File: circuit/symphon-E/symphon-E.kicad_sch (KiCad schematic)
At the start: 1 part

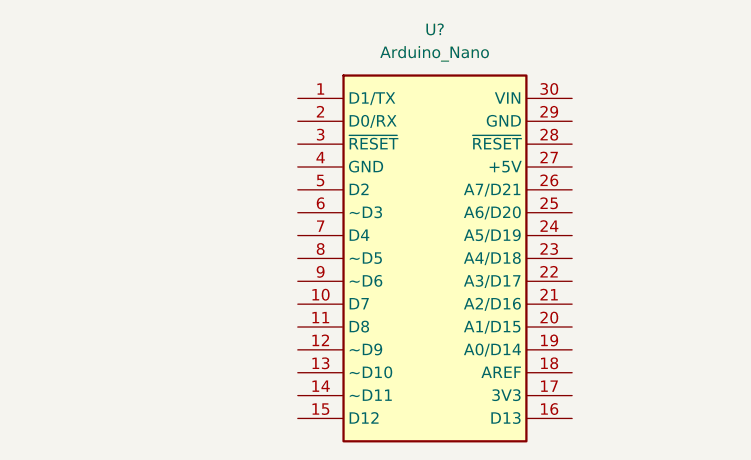
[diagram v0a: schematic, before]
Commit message: add pinout
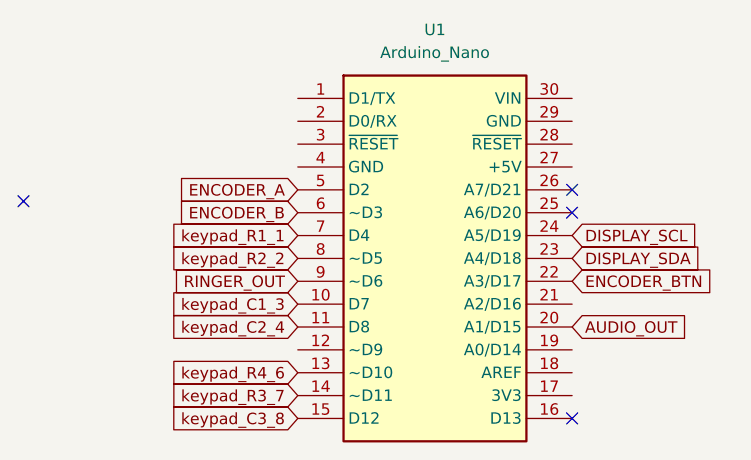
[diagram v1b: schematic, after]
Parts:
- gave numbers to parts that had none: 1
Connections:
- net keypad_C1_3: now reaches U1.10 (D7)
- net keypad_C2_4: now reaches U1.11 (D8)
- net keypad_R4_6: now reaches U1.13 (~D10)
- net keypad_R3_7: now reaches U1.14 (~D11)
- net keypad_C3_8: now reaches U1.15 (D12)
- net AUDIO_OUT: now reaches U1.20 (A1/D15)
- net ENCODER_BTN: now reaches U1.22 (A3/D17)
- net DISPLAY_SDA: now reaches U1.23 (A4/D18)
- net DISPLAY_SCL: now reaches U1.24 (A5/D19)
- net ENCODER_A: now reaches U1.5 (D2)
- net ENCODER_B: now reaches U1.6 (~D3)
- net keypad_R1_1: now reaches U1.7 (D4)
- net keypad_R2_2: now reaches U1.8 (~D5)
- net RINGER_OUT: now reaches U1.9 (~D6)
- no-connect marks 0 -> 4
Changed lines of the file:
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@@
 (kicad_sch (version 20211123) (generator eeschema)
   (paper "A4")
+  (no_connect (at 69.85 44.45))
+  (no_connect (at 8.89 43.18))
+  (no_connect (at 69.85 67.31))
+  (no_connect (at 69.85 41.91))
+  (global_label "ENCODER_A" (shape input) (at 39.37 41.91 180) (fields_autoplaced)
+    (effects (font (size 1.27 1.27)) (justify right))
+    (property "Intersheet References" "${INTERSHEET_REFS}" (id 0) (at 26.1317 41.8306 0)
+      (effects (font (size 1.27 1.27)) (justify right) hide)
+    )
+  )
+  (global_label "keypad_R2_2" (shape input) (at 39.37 49.53 180) (fields_autoplaced)
+    (effects (font (size 1.27 1.27)) (justify right))
+    (property "Intersheet References" "${INTERSHEET_REFS}" (id 0) (at 24.8012 49.4506 0)
+      (effects (font (size 1.27 1.27)) (justify right) hide)
+    )
+  )
+  (global_label "keypad_R4_6" (shape input) (at 39.37 62.23 180) (fields_autoplaced)
+    (effects (font (size 1.27 1.27)) (justify right))
+    (property "Intersheet References" "${INTERSHEET_REFS}" (id 0) (at 24.8012 62.1506 0)
+      (effects (font (size 1.27 1.27)) (justify right) hide)
+    )
+  )
+  (global_label "keypad_C2_4" (shape input) (at 39.37 57.15 180) (fields_autoplaced)
+    (effects (font (size 1.27 1.27)) (justify right))
+    (property "Intersheet References" "${INTERSHEET_REFS}" (id 0) (at 24.8012 57.0706 0)
+      (effects (font (size 1.27 1.27)) (justify right) hide)
+    )
+  )
+  (global_label "DISPLAY_SCL" (shape input) (at 69.85 46.99 0) (fields_autoplaced)
+    (effects (font (size 1.27 1.27)) (justify left))
+    (property "Intersheet References" "${INTERSHEET_REFS}" (id 0) (at 84.2979 46.9106 0)
+      (effects (font (size 1.27 1.27)) (justify left) hide)
+    )
+  )
+  (global_label "DISPLAY_SDA" (shape input) (at 69.85 49.53 0) (fields_autoplaced)
+    (effects (font (size 1.27 1.27)) (justify left))
+    (property "Intersheet References" "${INTERSHEET_REFS}" (id 0) (at 84.3583 49.4506 0)
+      (effects (font (size 1.27 1.27)) (justify left) hide)
+    )
+  )
+  (global_label "keypad_R1_1" (shape input) (at 39.37 46.99 180) (fields_autoplaced)
+    (effects (font (size 1.27 1.27)) (justify right))
+    (property "Intersheet References" "${INTERSHEET_REFS}" (id 0) (at 24.8012 46.9106 0)
+      (effects (font (size 1.27 1.27)) (justify right) hide)
+    )
+  )
+  (global_label "RINGER_OUT" (shape input) (at 39.37 52.07 180) (fields_autoplaced)
+    (effects (font (size 1.27 1.27)) (justify right))
+    (property "Intersheet References" "${INTERSHEET_REFS}" (id 0) (at 25.4664 51.9906 0)
+      (effects (font (size 1.27 1.27)) (justify right) hide)
+    )
+  )
+  (global_label "keypad_C1_3" (shape input) (at 39.37 54.61 180) (fields_autoplaced)
+    (effects (font (size 1.27 1.27)) (justify right))
+    (property "Intersheet References" "${INTERSHEET_REFS}" (id 0) (at 24.8012 54.5306 0)
+      (effects (font (size 1.27 1.27)) (justify right) hide)
+    )
+  )
+  (global_label "AUDIO_OUT" (shape input) (at 69.85 57.15 0) (fields_autoplaced)
+    (effects (font (size 1.27 1.27)) (justify left))
+    (property "Intersheet References" "${INTERSHEET_REFS}" (id 0) (at 82.4836 57.0706 0)
+      (effects (font (size 1.27 1.27)) (justify left) hide)
+    )
+  )
+  (global_label "ENCODER_B" (shape input) (at 39.37 44.45 180) (fields_autoplaced)
+    (effects (font (size 1.27 1.27)) (justify right))
+    (property "Intersheet References" "${INTERSHEET_REFS}" (id 0) (at 25.9502 44.3706 0)
+      (effects (font (size 1.27 1.27)) (justify right) hide)
+    )
+  )
+  (global_label "ENCODER_BTN" (shape input) (at 69.85 52.07 0) (fields_autoplaced)
+    (effects (font (size 1.27 1.27)) (justify left))
+    (property "Intersheet References" "${INTERSHEET_REFS}" (id 0) (at 85.5679 51.9906 0)
+      (effects (font (size 1.27 1.27)) (justify left) hide)
+    )
+  )
+  (global_label "keypad_R3_7" (shape input) (at 39.37 64.77 180) (fields_autoplaced)
+    (effects (font (size 1.27 1.27)) (justify right))
+    (property "Intersheet References" "${INTERSHEET_REFS}" (id 0) (at 24.8012 64.6906 0)
+      (effects (font (size 1.27 1.27)) (justify right) hide)
+    )
+  )
+  (global_label "keypad_C3_8" (shape input) (at 39.37 67.31 180) (fields_autoplaced)
+    (effects (font (size 1.27 1.27)) (justify right))
+    (property "Intersheet References" "${INTERSHEET_REFS}" (id 0) (at 24.8012 67.2306 0)
+      (effects (font (size 1.27 1.27)) (justify right) hide)
+    )
+  )
   (symbol (lib_id "Arduino:Arduino_Nano") (at 54.61 49.53 0) (unit 1)
     (in_bom yes) (on_board yes) (fields_autoplaced)
-    (property "Reference" "U?" (id 0) (at 54.61 24.13 0))
+    (property "Reference" "U1" (id 0) (at 54.61 24.13 0))
     (property "Value" "Arduino_Nano" (id 1) (at 54.61 26.67 0))
     (property "Footprint" "Arduino:Arduino_Nano" (id 2) (at 54.61 71.12 0)
@@
   (symbol_instances
     (path "/05df8035-1ae4-4fd6-8683-6c4f92e2cd4b"
-      (reference "U?") (unit 1) (value "Arduino_Nano") (footprint "Arduino:Arduino_Nano")
+      (reference "U1") (unit 1) (value "Arduino_Nano") (footprint "Arduino:Arduino_Nano")
     )
   )

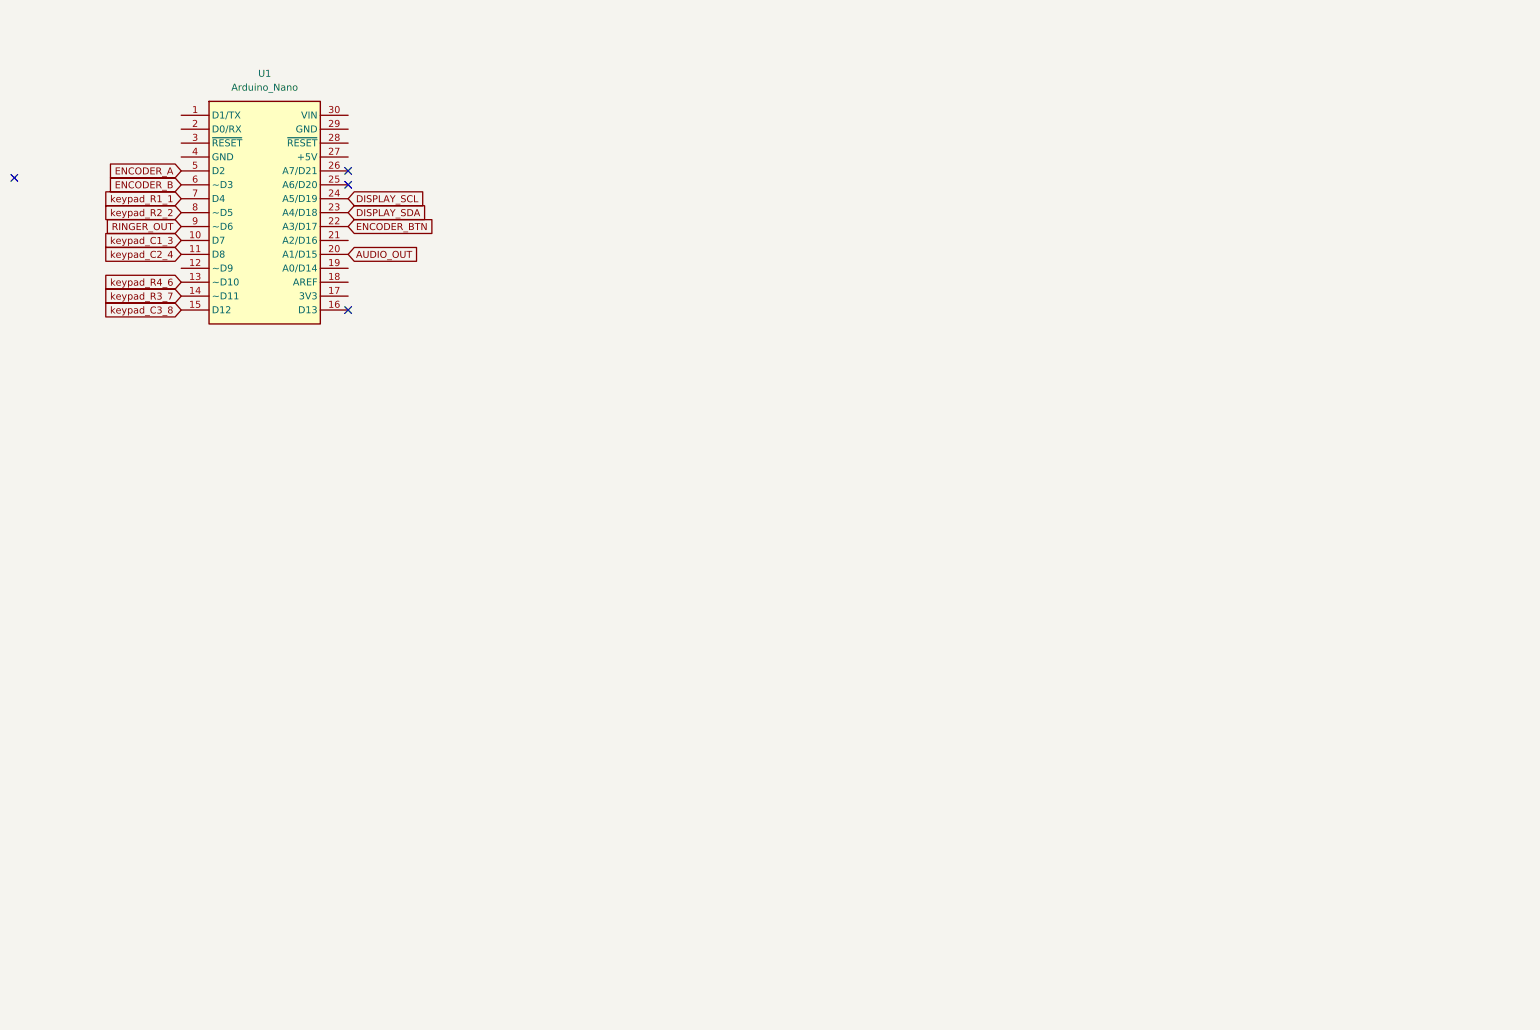
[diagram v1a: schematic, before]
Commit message: add pcb
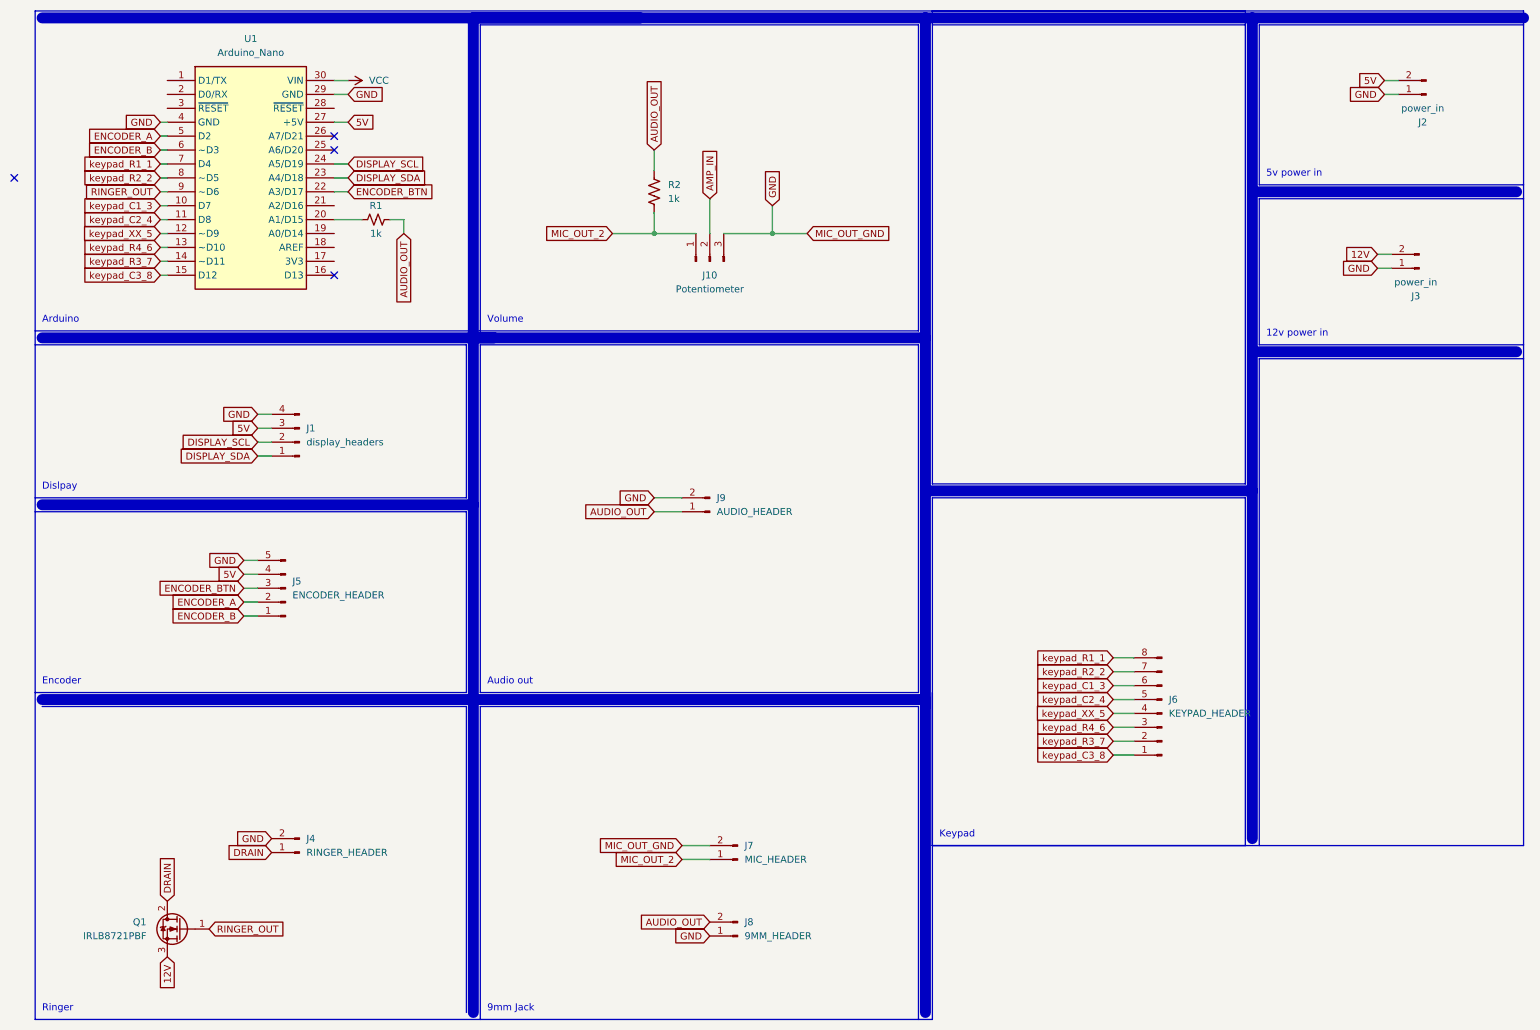
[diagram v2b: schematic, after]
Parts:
- added J1: display_headers, Connector_JST:JST_EH_B4B-EH-A_1x04_P2.50mm_Vertical, symbol Connector:Conn_01x04_Male
- added J10: Potentiometer, Connector_JST:JST_EH_B3B-EH-A_1x03_P2.50mm_Vertical, symbol Connector:Conn_01x03_Male
- added J2, J3: power_in, Connector_JST:JST_EH_B2B-EH-A_1x02_P2.50mm_Vertical, symbol Connector:Conn_01x02_Male
- added J4: RINGER_HEADER, Connector_JST:JST_EH_B2B-EH-A_1x02_P2.50mm_Vertical, symbol Connector:Conn_01x02_Male
- added J5: ENCODER_HEADER, Connector_JST:JST_EH_B5B-EH-A_1x05_P2.50mm_Vertical, symbol Connector:Conn_01x05_Male
- added J6: KEYPAD_HEADER, Connector_JST:JST_EH_B8B-EH-A_1x08_P2.50mm_Vertical, symbol Connector:Conn_01x08_Male
- added J7: MIC_HEADER, Connector_JST:JST_EH_B2B-EH-A_1x02_P2.50mm_Vertical, symbol Connector:Conn_01x02_Male
- added J8: 9MM_HEADER, Connector_JST:JST_EH_B2B-EH-A_1x02_P2.50mm_Vertical, symbol Connector:Conn_01x02_Male
- added J9: AUDIO_HEADER, Connector_JST:JST_EH_B2B-EH-A_1x02_P2.50mm_Vertical, symbol Connector:Conn_01x02_Male
- added Q1: IRLB8721PBF, Package_TO_SOT_THT:TO-220-3_Vertical, symbol Transistor_FET:IRLB8721PBF
- added R1: 1k, Resistor_THT:R_Axial_DIN0204_L3.6mm_D1.6mm_P7.62mm_Horizontal, symbol Device:R_Small_US
- added R2: 1k, Resistor_THT:R_Axial_DIN0204_L3.6mm_D1.6mm_P7.62mm_Horizontal, symbol Device:R_US
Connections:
- net AUDIO_OUT: now also J8.2 (Pin_2), J9.1 (Pin_1), R1.2, R2.1; no longer U1.20 (A1/D15)
- net DISPLAY_SCL: now also J1.2 (Pin_2)
- net DISPLAY_SDA: now also J1.1 (Pin_1)
- net ENCODER_A: now also J5.2 (Pin_2)
- net ENCODER_B: now also J5.1 (Pin_1)
- net ENCODER_BTN: now also J5.3 (Pin_3)
- net RINGER_OUT: now also Q1.1 (G)
- net keypad_C1_3: now also J6.6 (Pin_6)
- net keypad_C2_4: now also J6.5 (Pin_5)
- net keypad_C3_8: now also J6.1 (Pin_1)
- net keypad_R1_1: now also J6.8 (Pin_8)
- net keypad_R2_2: now also J6.7 (Pin_7)
- net keypad_R3_7: now also J6.2 (Pin_2)
- net keypad_R4_6: now also J6.3 (Pin_3)
- net keypad_XX_5: now reaches U1.12 (~D9)
- net keypad_XX_5: now also J6.4 (Pin_4)
- net 5V: now reaches U1.27 (+5V)
- net 5V: now also J1.3 (Pin_3), J2.2 (Pin_2), J5.4 (Pin_4)
- net GND: now reaches U1.29 (GND)
- net GND: now also U1.4 (GND), J1.4 (Pin_4), J10.3 (Pin_3), J2.1 (Pin_1), J3.1 (Pin_1), J4.2 (Pin_2), J5.5 (Pin_5), J7.2 (Pin_2), J8.1 (Pin_1), J9.2 (Pin_2)
- net VCC: now reaches U1.30 (VIN)
- new net: R1.1, U1.20 (A1/D15)
- new net 12V: J3.2 (Pin_2), Q1.3 (S)
- new net AMP_IN: J10.2 (Pin_2)
- new net DRAIN: J4.1 (Pin_1), Q1.2 (D)
- new net MIC_OUT_2: J10.1 (Pin_1), J7.1 (Pin_1), R2.2
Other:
- note added: "12v power in"
- note added: "5v power in"
- note added: "9mm Jack"
- note added: "Arduino"
- note added: "Audio out"
- note added: "Dislpay"
- note added: "Encoder"
- note added: "Keypad"
- note added: "Ringer"
- note added: "Volume"
- moved on the sheet: U1
